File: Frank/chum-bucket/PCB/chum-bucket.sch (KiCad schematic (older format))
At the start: 3 parts

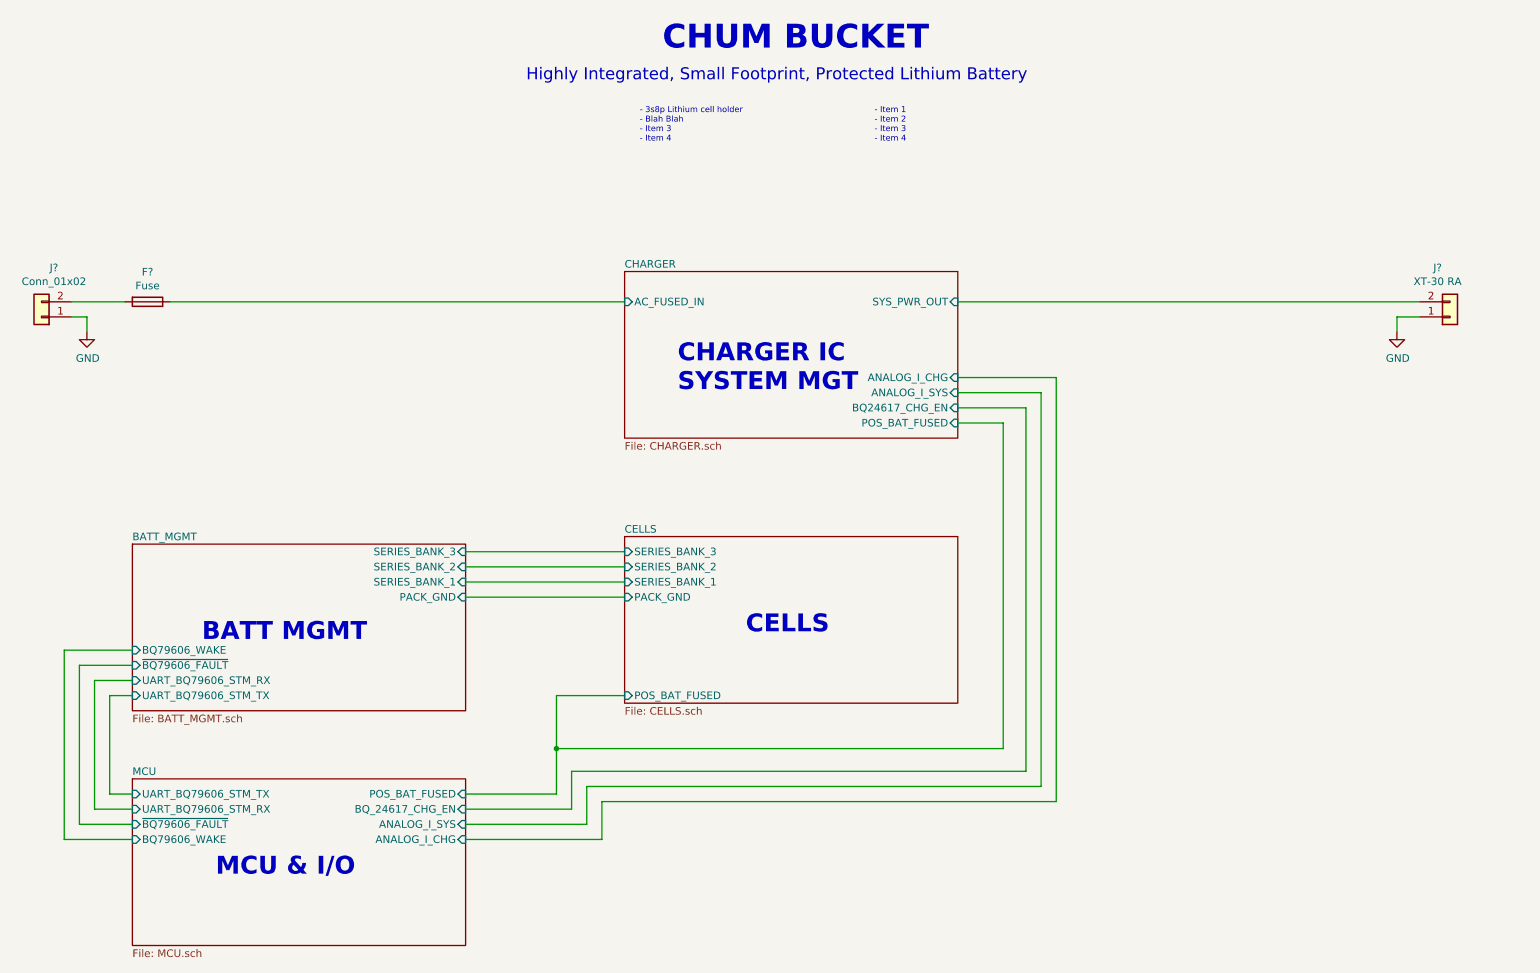
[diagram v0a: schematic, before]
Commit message: Weekends work. Final component selection then ready for review :)
huge oof
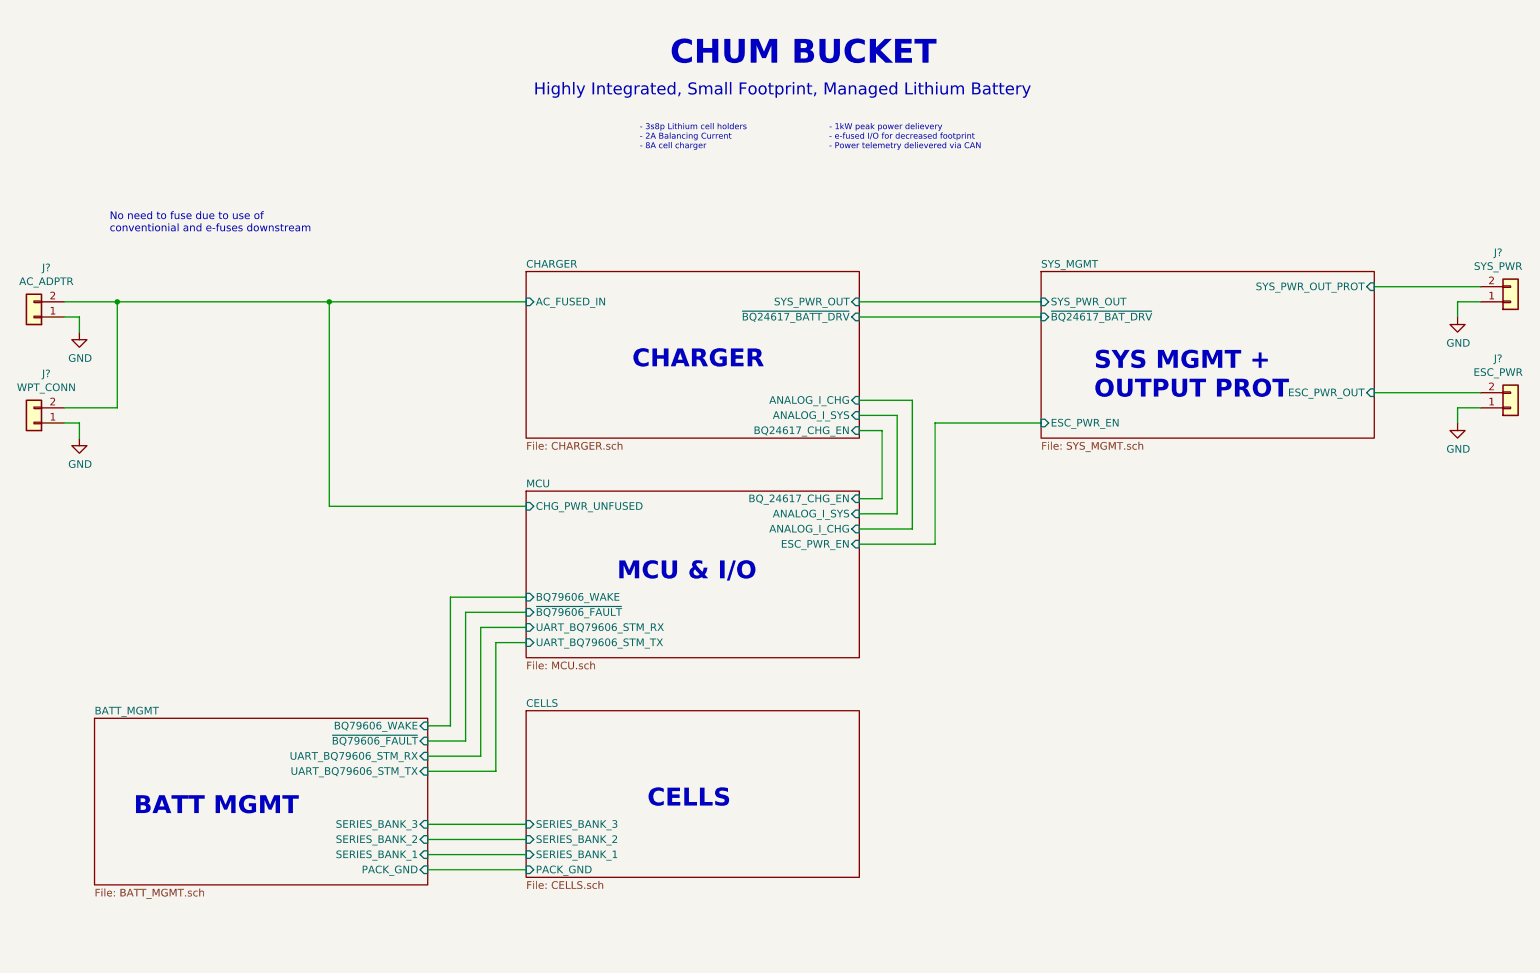
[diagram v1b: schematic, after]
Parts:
- removed F?: Fuse, symbol Device:Fuse
- removed J?: XT-30 RA, symbol Connector_Generic:Conn_01x02
- added J?: WPT_CONN, symbol Connector_Generic:Conn_01x02
- added J?: SYS_PWR, symbol Connector_Generic:Conn_01x02
- added J?: ESC_PWR, symbol Connector_Generic:Conn_01x02
- J?: value Conn_01x02 -> AC_ADPTR
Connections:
- net CHARGER/AC_FUSED_IN: now also J?.2 (Pin_2), J?.2 (Pin_2)
- net GND: now also J?.1 (Pin_1), J?.1 (Pin_1), J?.1 (Pin_1)
- new net SYS_MGMT/ESC_PWR_OUT: J?.2 (Pin_2)
- new net SYS_MGMT/SYS_PWR_OUT_PROT: J?.2 (Pin_2)
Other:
- note added: "- 1kW peak power delievery\n- e-fused I/O for decreased footprint\n- Power telemetry delievered via CAN"
- note added: "- 3s8p Lithium cell holders\n- 2A Balancing Current\n- 8A cell charger"
- note added: "CHARGER"
- note added: "Highly Integrated, Small Footprint, Managed Lithium Battery"
- note added: "No need to fuse due to use of \nconventionial and e-fuses downstream"
- note added: "SYS MGMT +\nOUTPUT PROT"
- note removed: "- 3s8p Lithium cell holder\n- Blah Blah\n- Item 3\n- Item 4"
- note removed: "- Item 1\n- Item 2\n- Item 3\n- Item 4"
- note removed: "CHARGER IC\nSYSTEM MGT"
- note removed: "Highly Integrated, Small Footprint, Protected Lithium Battery"
- moved on the sheet: J?
